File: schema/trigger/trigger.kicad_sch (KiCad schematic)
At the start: 28 parts, among them IC1 RP2040_ZERO, IC2 SSD1306, J1 Barrel_Jack, J2 Conn_01x02_Socket, J3 Conn_01x02_Pin, J4 Conn_01x04_Pin, Q1 DMG4800LK3-13, SW1 SW_Push

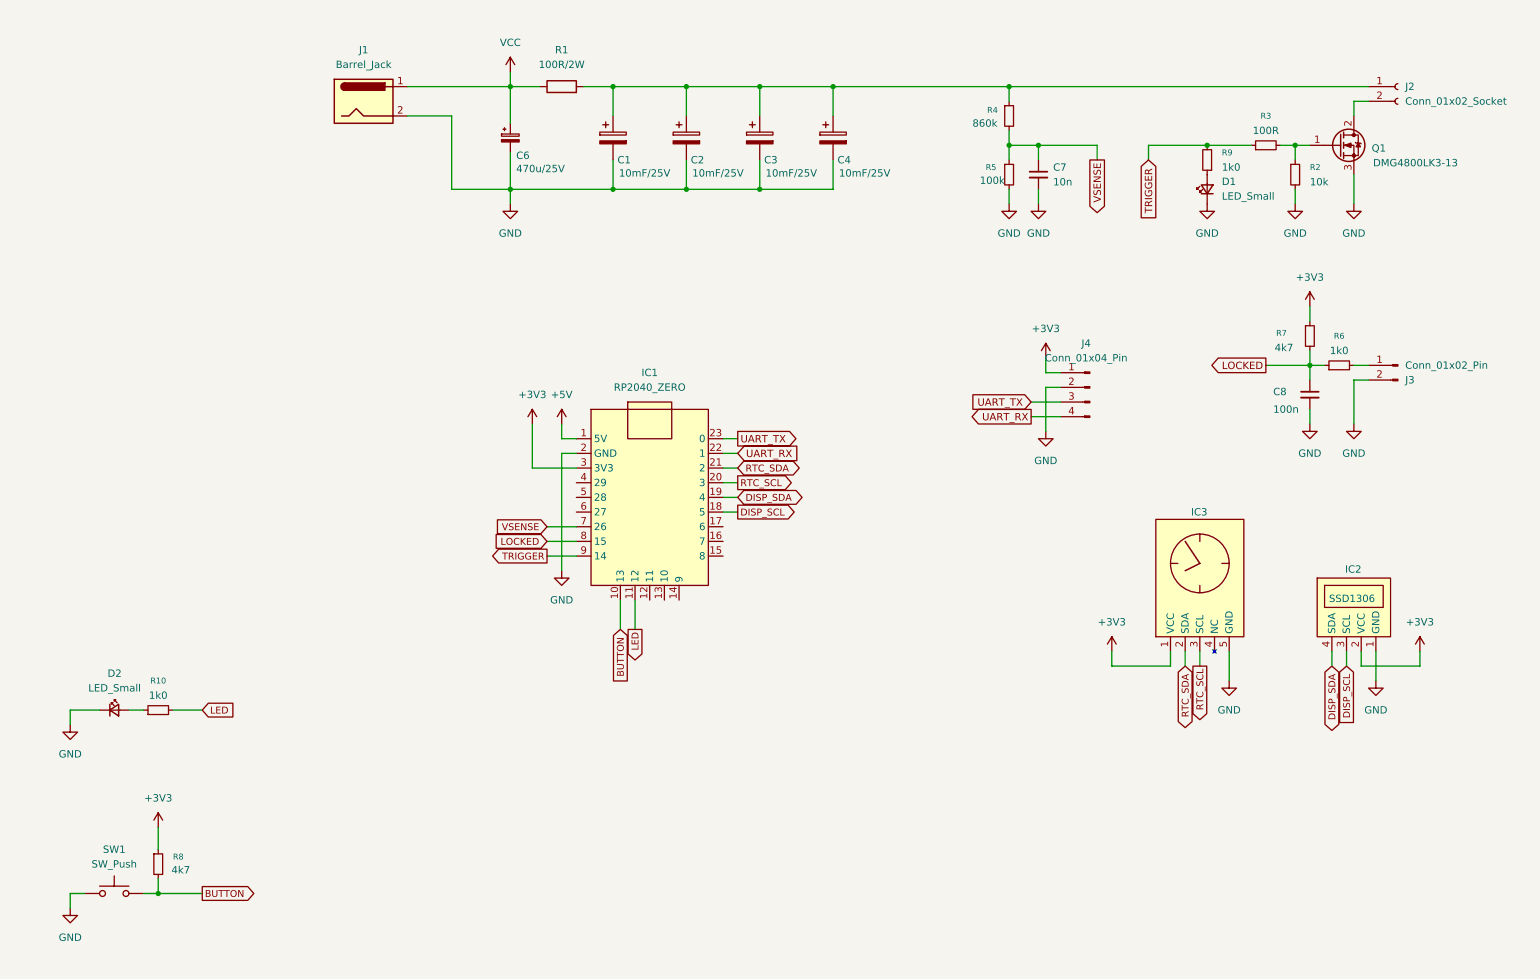
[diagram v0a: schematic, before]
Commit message: pcb design
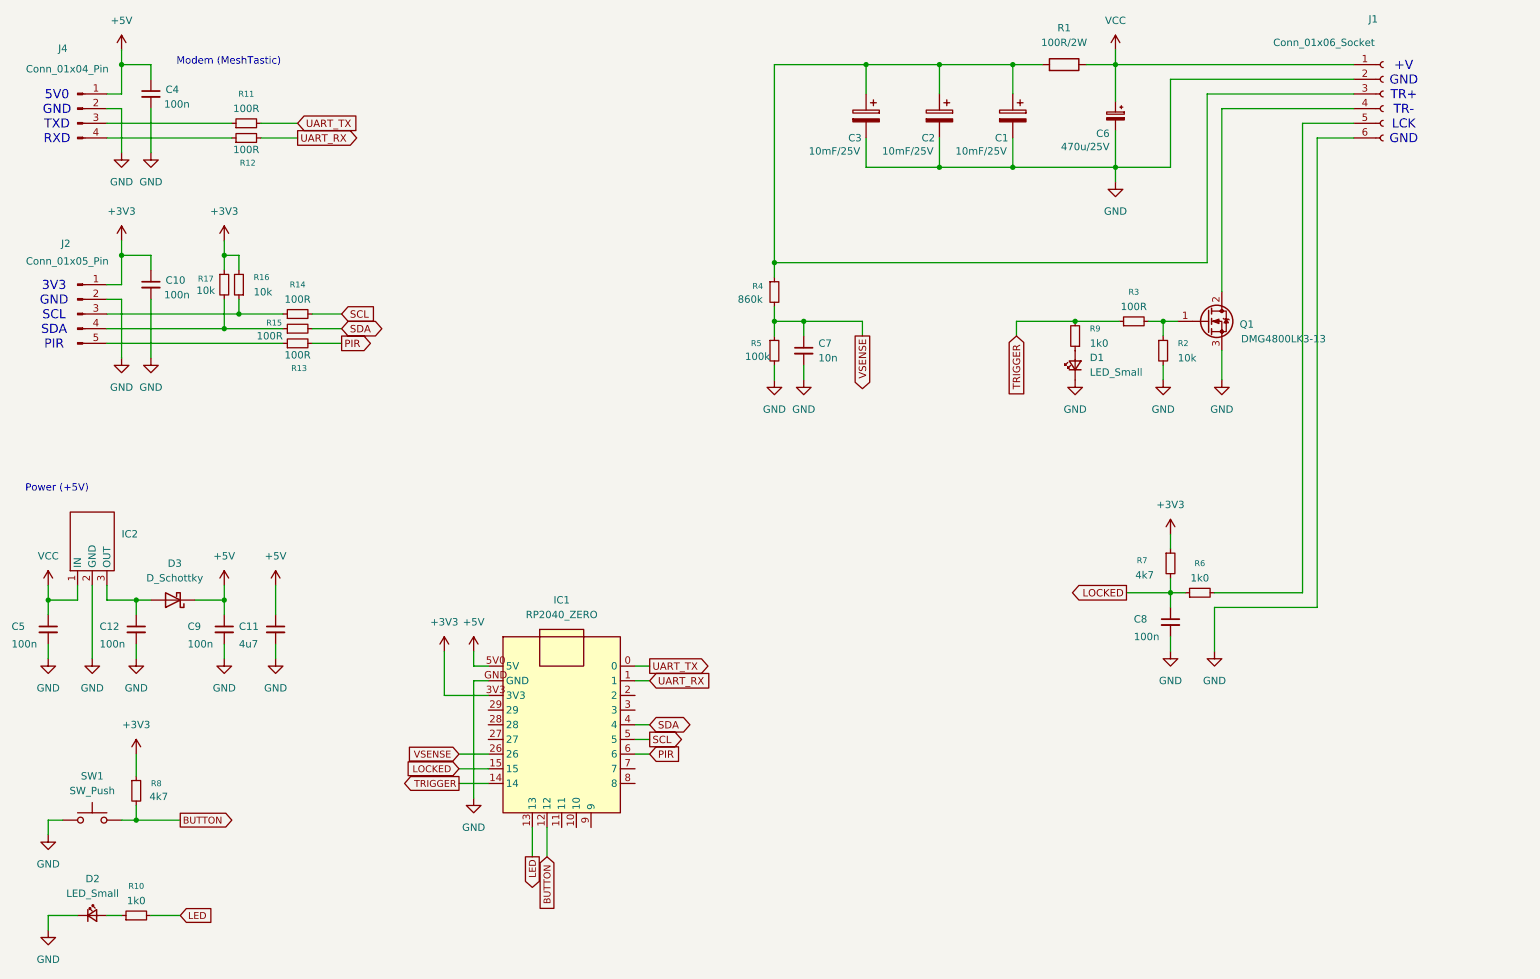
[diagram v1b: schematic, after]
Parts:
- removed C4: 10mF/25V, myLibrary:C_36x18, symbol Device:C_Polarized
- removed IC2: SSD1306, myLibrary:OLED_I2C_128x64_SMD, symbol mySymbols:OLED_I2C
- removed IC3: ~, symbol mySymbols:RTC
- removed J1: Barrel_Jack, Connector_BarrelJack:BarrelJack_GCT_DCJ200-10-A_Horizontal, symbol Connector:Barrel_Jack
- removed J2: Conn_01x02_Socket, symbol Connector:Conn_01x02_Socket
- removed J3: Conn_01x02_Pin, symbol Connector:Conn_01x02_Pin
- added C10, C12, C4, C5, C9: 100n, Capacitor_SMD:C_0603_1608Metric, symbol Device:C_Small
- added C11: 4u7, Capacitor_SMD:C_1206_3216Metric, symbol Device:C_Small
- added D3: D_Schottky, Diode_SMD:D_SOD-123F, symbol Device:D_Schottky
- added IC2: ~, myLibrary:Untitled_3, symbol mySymbols:VoltageReg
- added J1: Conn_01x06_Socket, myLibrary:Solder_Terminal_6p, symbol Connector:Conn_01x06_Socket
- added J2: Conn_01x05_Pin, myLibrary:Solder_Terminal_5p, symbol Connector:Conn_01x05_Pin
- added R11, R12, R13, R14, R15: 100R, Resistor_SMD:R_0603_1608Metric, symbol Device:R_Small
- added R16, R17: 10k, Resistor_SMD:R_0603_1608Metric, symbol Device:R_Small
- IC1: footprint (none) -> myLibrary:RP2040_ZERO
- J4: footprint (none) -> myLibrary:Solder_Terminal_4p
- SW1: footprint (none) -> Button_Switch_SMD:SW_SPST_SKQG_WithStem
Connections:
- net +3V3: now also IC1.3V3, C10.1, J2.1 (Pin_1), R16.2, R17.1; no longer IC1.3 (3V3), J4.1 (Pin_1)
- net +5V: now also IC1.5V0 (5V), J4.1 (Pin_1), C11.1, C4.1, C9.1, D3.1 (K); no longer IC1.1 (5V)
- net BUTTON: now also IC1.12; no longer IC1.10 (13)
- net GND: now also IC1.GND, C10.2, C11.2, C12.2, C4.2, C5.2, C9.2, IC2.2 (GND), J1.2 (Pin_2), J1.6 (Pin_6), J2.2 (Pin_2); no longer IC1.2 (GND)
- net LED: now also IC1.13; no longer IC1.11 (12)
- net LOCKED: now also IC1.15; no longer IC1.8 (15)
- net TRIGGER: now also IC1.14; no longer IC1.9 (14)
- net UART_RX: now also IC1.1, R12.2; no longer IC1.22 (1), J4.4 (Pin_4)
- net UART_TX: now also IC1.0, R11.2; no longer IC1.23 (0), J4.3 (Pin_3)
- net VCC: now also C5.1, IC2.1 (IN), J1.1 (Pin_1)
- net VSENSE: now also IC1.26; no longer IC1.7 (26)
- net at Q1.2 (D): now also J1.4 (Pin_4)
- net at R6.2: now also J1.5 (Pin_5)
- net at C1.1, C2.1, C3.1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: now also J1.3 (Pin_3)
- net SDA: now reaches IC1.4
- net SDA: now also R15.2
- net SCL: now reaches IC1.5
- net SCL: now also R14.2
- net PIR: now reaches IC1.6
- net PIR: now also R13.2
- removed net DISP_SCL: IC1.18 (5)
- removed net DISP_SDA: IC1.19 (4)
- removed net RTC_SCL: IC1.20 (3)
- removed net RTC_SDA: IC1.21 (2)
- new net: J2.3 (Pin_3), R14.1, R16.1
- new net: J2.4 (Pin_4), R15.1, R17.2
- new net: J2.5 (Pin_5), R13.1
- new net: C12.1, D3.2 (A), IC2.3 (OUT)
- new net: J4.4 (Pin_4), R12.1
- new net: J4.3 (Pin_3), R11.1
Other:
- note added: "+V GND TR+ TR- LCK GND"
- note added: "3V3 GND SCL SDA PIR"
- note added: "5V0 GND TXD RXD"
- note added: "Modem (MeshTastic)"
- note added: "Power (+5V)"
- moved on the sheet: C1, C2, C3, C6, C7, C8, D1, D2, IC1, J4, Q1, R1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
